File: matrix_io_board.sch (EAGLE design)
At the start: 114 parts, among them IC1 6N138, IC2 SN74LVC2G14, IC3 LM27675M5_CHARGEPUMP, IC4 LM324D, IC5 MCP4728_QUAD_DAC, IC6 4504D, IC7 SP34063A_BOOST_REG, IC8 FDS8958B

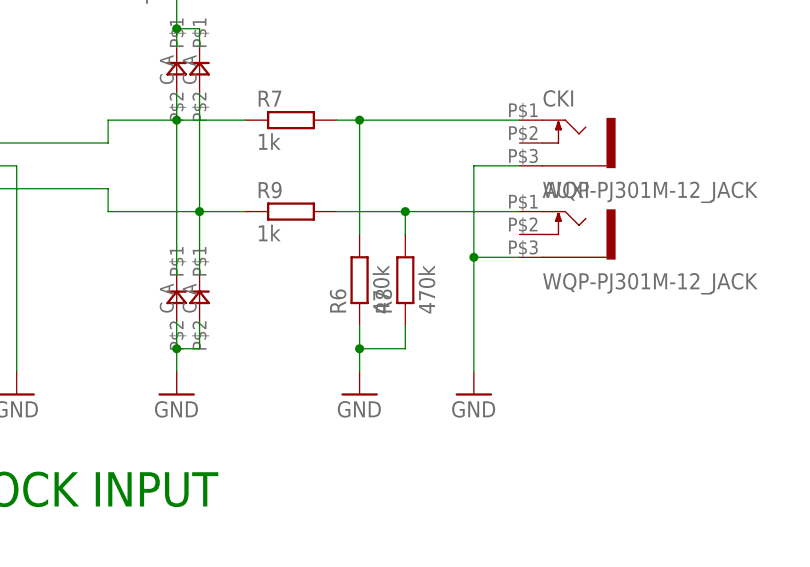
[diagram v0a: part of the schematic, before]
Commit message: values
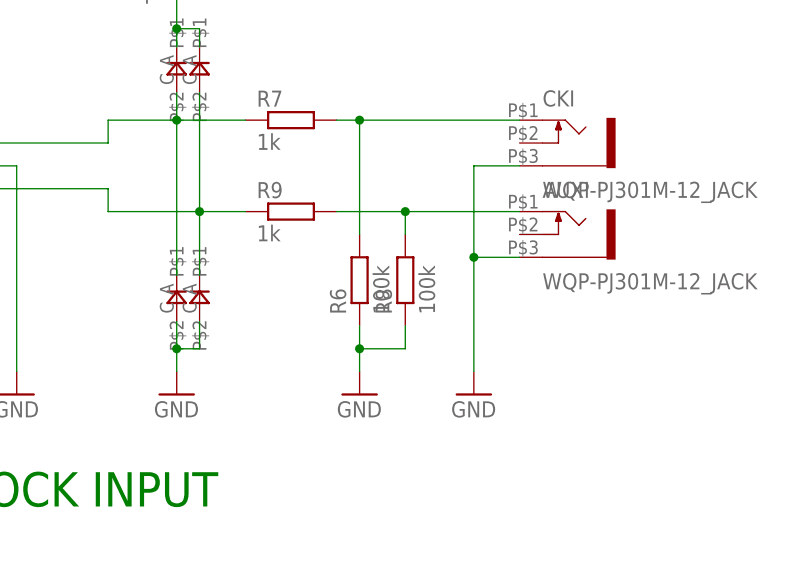
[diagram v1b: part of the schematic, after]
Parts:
- R6, R8: value 470k -> 100k
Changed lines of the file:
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@@
 <part name="5V." library="pinhead" deviceset="PINHD-1X1" device=""/>
 <part name="OFFSW" library="pinhead" deviceset="PINHD-1X1" device=""/>
-<part name="R6" library="rcl" deviceset="R-EU_" device="R0805" value="470k"/>
+<part name="R6" library="rcl" deviceset="R-EU_" device="R0805" value="100k"/>
 <part name="GND26" library="supply1" deviceset="GND" device=""/>
 <part name="C5" library="rcl" deviceset="C-EU" device="C0805" value="100n"/>
@@
 <part name="R9" library="rcl" deviceset="R-EU_" device="R0805" value="1k"/>
 <part name="GND20" library="supply1" deviceset="GND" device=""/>
-<part name="R8" library="rcl" deviceset="R-EU_" device="R0805" value="470k"/>
+<part name="R8" library="rcl" deviceset="R-EU_" device="R0805" value="100k"/>
 <part name="D4" library="jasons_stuff" deviceset="0805DIODE" device=""/>
 <part name="D5" library="jasons_stuff" deviceset="0805DIODE" device=""/>
